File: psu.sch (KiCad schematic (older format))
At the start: 64 parts, among them J1 Screw_Terminal_01x02, J2 Barrel_Jack, J3 Binding posts, SW1 SW_SP4T, SW2 SW_SP4T, SW3 Lever toggle, U1 LM4040DBZ-2.5, U2 LT3081, U3 LM393, U4 LM334M, U5 LM317L_TO92, U6 LM317L_TO92

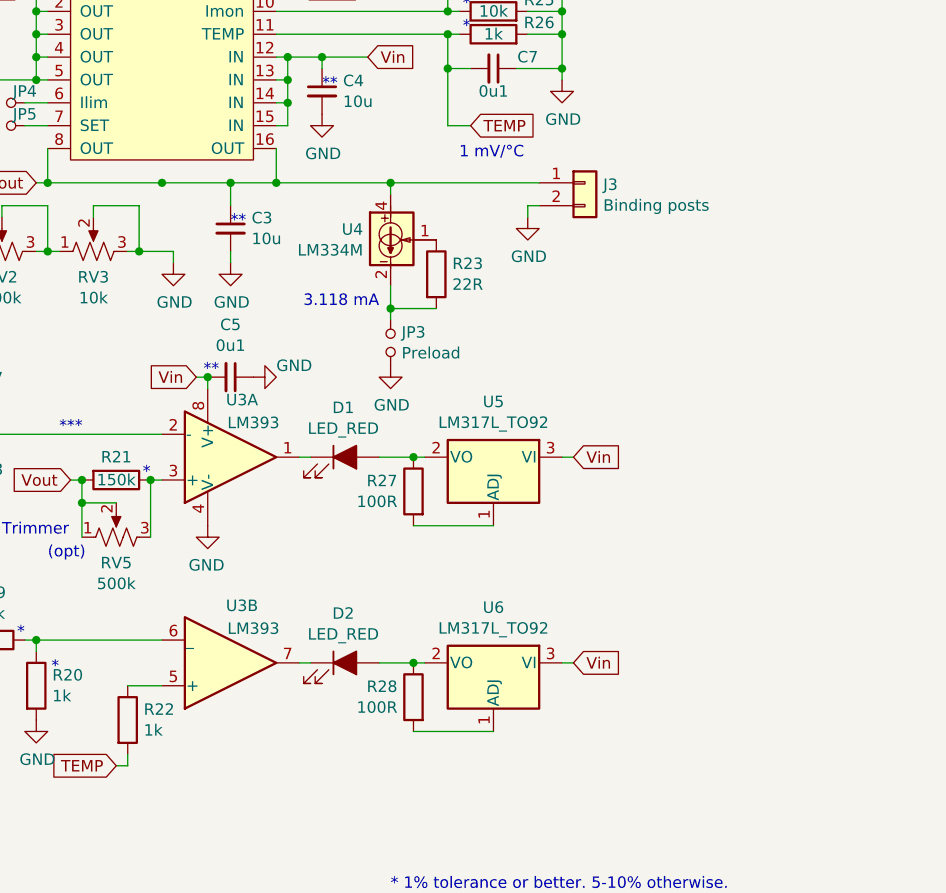
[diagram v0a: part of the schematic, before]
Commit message: More routing; some issues
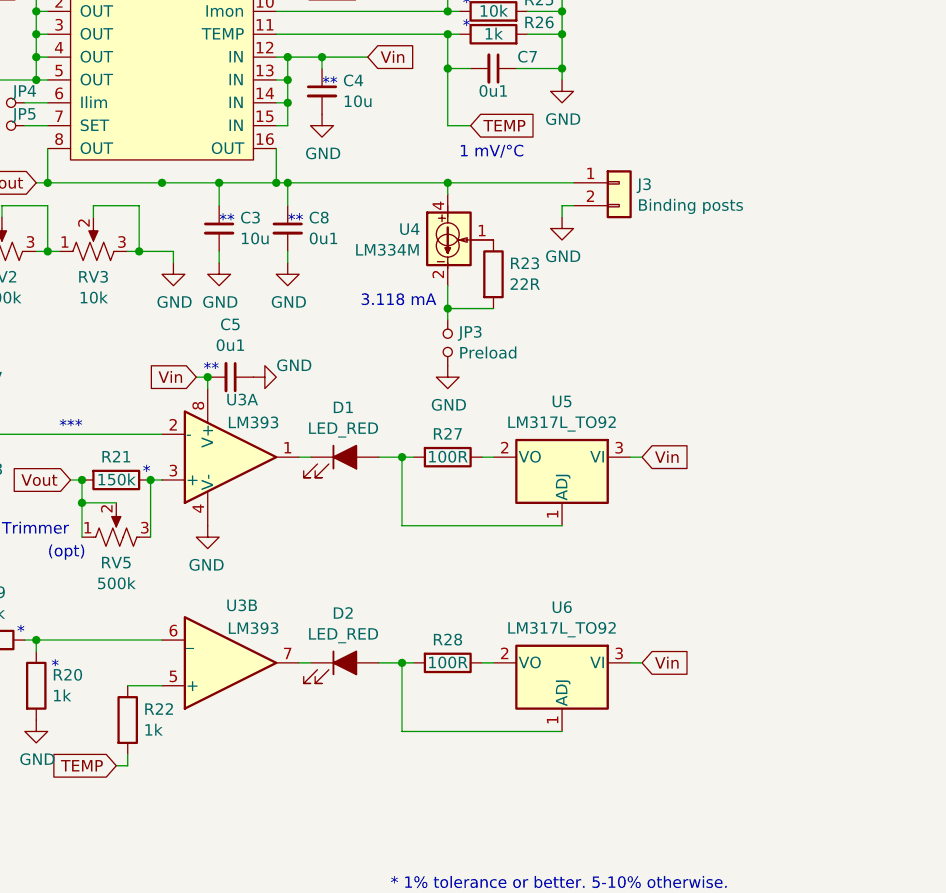
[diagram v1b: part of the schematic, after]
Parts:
- added C8: 0u1, Capacitor_THT:C_Disc_D5.0mm_W2.5mm_P2.50mm, symbol Device:C_Small
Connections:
- net GND: now also C8.2
- net Vout: now also C8.1
- net at R27.2, U5.1 (ADJ): now also D1.2 (A)
- net at R27.1, U5.2 (VO): no longer D1.2 (A)
- net at R28.2, U6.1 (ADJ): now also D2.2 (A)
- net at R28.1, U6.2 (VO): no longer D2.2 (A)
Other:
- moved on the sheet: C3, J3, JP3, R23, U4, U5

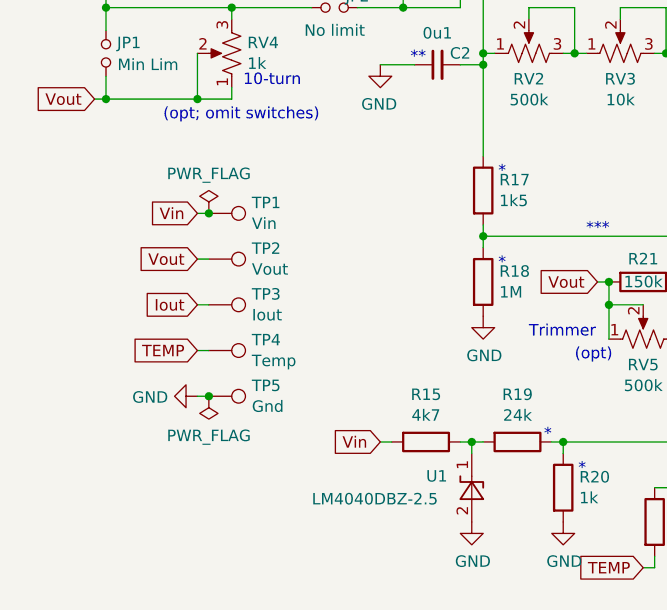
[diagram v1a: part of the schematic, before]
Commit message: It's all connected man
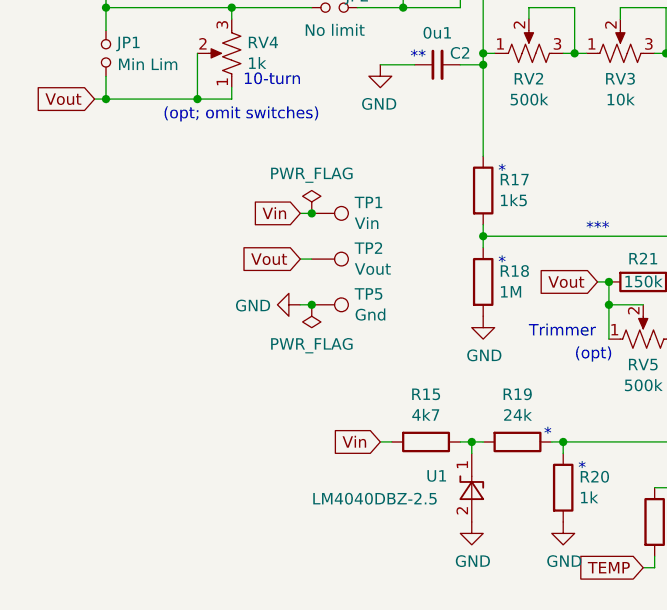
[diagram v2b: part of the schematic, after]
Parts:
- removed TP3: Iout, TestPoint:TestPoint_Bridge_Pitch2.54mm_Drill1.3mm, symbol Connector:TestPoint
- removed TP4: Temp, TestPoint:TestPoint_Bridge_Pitch2.54mm_Drill1.3mm, symbol Connector:TestPoint
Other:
- moved on the sheet: TP1, TP2, TP5
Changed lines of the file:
@@
 Wire Wire Line
 	7750 3650 7800 3650
-Text GLabel 3850 4550 0    50   Input ~ 0
+Text GLabel 4300 4550 0    50   Input ~ 0
 Vin
 Wire Wire Line
-	3850 4550 3900 4550
-Text GLabel 3850 5150 0    50   Input ~ 0
-TEMP
-Text GLabel 3850 4950 0    50   Input ~ 0
-Iout
-Text GLabel 3850 4750 0    50   Input ~ 0
+	4300 4550 4350 4550
+Text GLabel 4300 4750 0    50   Input ~ 0
 Vout
 Wire Wire Line
-	3850 4750 3900 4750
-Wire Wire Line
-	3900 4950 3850 4950
-Wire Wire Line
-	3850 5150 3900 5150
+	4300 4750 4350 4750
 Connection ~ 5100 3850
 $Comp
@@
 L Connector:TestPoint TP2
 U 1 1 5D1B06FD
-P 3900 4750
-F 0 "TP2" V 3854 4938 50  0000 L CNN
-F 1 "Vout" V 3945 4938 50  0000 L CNN
-F 2 "TestPoint:TestPoint_Bridge_Pitch2.54mm_Drill1.3mm" H 4100 4750 50  0001 C CNN
-F 3 "~" H 4100 4750 50  0001 C CNN
-	1    3900 4750
-	0    1    1    0
-$EndComp
-$Comp
-L Connector:TestPoint TP3
-U 1 1 5D1BB2CF
-P 3900 4950
-F 0 "TP3" V 3854 5138 50  0000 L CNN
-F 1 "Iout" V 3945 5138 50  0000 L CNN
-F 2 "TestPoint:TestPoint_Bridge_Pitch2.54mm_Drill1.3mm" H 4100 4950 50  0001 C CNN
-F 3 "~" H 4100 4950 50  0001 C CNN
-	1    3900 4950
-	0    1    1    0
-$EndComp
-$Comp
-L Connector:TestPoint TP4
-U 1 1 5D1BFE83
-P 3900 5150
-F 0 "TP4" V 3854 5338 50  0000 L CNN
-F 1 "Temp" V 3945 5338 50  0000 L CNN
-F 2 "TestPoint:TestPoint_Bridge_Pitch2.54mm_Drill1.3mm" H 4100 5150 50  0001 C CNN
-F 3 "~" H 4100 5150 50  0001 C CNN
-	1    3900 5150
+P 4350 4750
+F 0 "TP2" V 4304 4938 50  0000 L CNN
+F 1 "Vout" V 4395 4938 50  0000 L CNN
+F 2 "TestPoint:TestPoint_Bridge_Pitch2.54mm_Drill1.3mm" H 4550 4750 50  0001 C CNN
+F 3 "~" H 4550 4750 50  0001 C CNN
+	1    4350 4750
 	0    1    1    0
 $EndComp
@@
 L Connector:TestPoint TP1
 U 1 1 5D1C006B
-P 3900 4550
-F 0 "TP1" V 3854 4738 50  0000 L CNN
-F 1 "Vin" V 3945 4738 50  0000 L CNN
-F 2 "TestPoint:TestPoint_Bridge_Pitch2.54mm_Drill1.3mm" H 4100 4550 50  0001 C CNN
-F 3 "~" H 4100 4550 50  0001 C CNN
-	1    3900 4550
-	0    1    1    0
-$EndComp
-$Comp
-L power:GND #PWR01
-U 1 1 5D1D360C
-P 3850 5350
-F 0 "#PWR01" H 3850 5100 50  0001 C CNN
-F 1 "GND" V 3855 5222 50  0000 R CNN
-F 2 "" H 3850 5350 50  0001 C CNN
-F 3 "" H 3850 5350 50  0001 C CNN
-	1    3850 5350
-	0    1    1    0
-$EndComp
-Wire Wire Line
-	3850 5350 3900 5350
+P 4350 4550
+F 0 "TP1" V 4304 4738 50  0000 L CNN
+F 1 "Vin" V 4395 4738 50  0000 L CNN
+F 2 "TestPoint:TestPoint_Bridge_Pitch2.54mm_Drill1.3mm" H 4550 4550 50  0001 C CNN
+F 3 "~" H 4550 4550 50  0001 C CNN
+	1    4350 4550
+	0    1    1    0
+$EndComp
+Wire Wire Line
+	4300 4950 4350 4950
 $Comp
 L Connector:TestPoint TP5
 U 1 1 5D1D96AA
-P 3900 5350
-F 0 "TP5" V 3854 5538 50  0000 L CNN
-F 1 "Gnd" V 3945 5538 50  0000 L CNN
-F 2 "TestPoint:TestPoint_Bridge_Pitch2.54mm_Drill1.3mm" H 4100 5350 50  0001 C CNN
-F 3 "~" H 4100 5350 50  0001 C CNN
-	1    3900 5350
+P 4350 4950
+F 0 "TP5" V 4304 5138 50  0000 L CNN
+F 1 "Gnd" V 4395 5138 50  0000 L CNN
+F 2 "TestPoint:TestPoint_Bridge_Pitch2.54mm_Drill1.3mm" H 4550 4950 50  0001 C CNN
+F 3 "~" H 4550 4950 50  0001 C CNN
+	1    4350 4950
 	0    1    1    0
 $EndComp
@@
 L power:PWR_FLAG #FLG01
 U 1 1 5D1E24E0
-P 3900 4550
-F 0 "#FLG01" H 3900 4625 50  0001 C CNN
-F 1 "PWR_FLAG" H 3900 4723 50  0000 C CNN
-F 2 "" H 3900 4550 50  0001 C CNN
-F 3 "~" H 3900 4550 50  0001 C CNN
-	1    3900 4550
-	1    0    0    -1
-$EndComp
-Connection ~ 3900 4550
+P 4350 4550
+F 0 "#FLG01" H 4350 4625 50  0001 C CNN
+F 1 "PWR_FLAG" H 4350 4723 50  0000 C CNN
+F 2 "" H 4350 4550 50  0001 C CNN
+F 3 "~" H 4350 4550 50  0001 C CNN
+	1    4350 4550
+	1    0    0    -1
+$EndComp
+Connection ~ 4350 4550
 $Comp
 L power:PWR_FLAG #FLG02
 U 1 1 5D1E310A
-P 3900 5350
-F 0 "#FLG02" H 3900 5425 50  0001 C CNN
-F 1 "PWR_FLAG" H 3900 5523 50  0000 C CNN
-F 2 "" H 3900 5350 50  0001 C CNN
-F 3 "~" H 3900 5350 50  0001 C CNN
-	1    3900 5350
+P 4350 4950
+F 0 "#FLG02" H 4350 5025 50  0001 C CNN
+F 1 "PWR_FLAG" H 4350 5123 50  0000 C CNN
+F 2 "" H 4350 4950 50  0001 C CNN
+F 3 "~" H 4350 4950 50  0001 C CNN
+	1    4350 4950
 	-1   0    0    1
 $EndComp
-Connection ~ 3900 5350
+Connection ~ 4350 4950
 Wire Wire Line
 	5050 5550 5100 5550
@@
 Wire Wire Line
 	7050 5650 7100 5650
+$Comp
+L power:GND #PWR01
+U 1 1 5D1D360C
+P 4300 4950
+F 0 "#PWR01" H 4300 4700 50  0001 C CNN
+F 1 "GND" V 4305 4822 50  0000 R CNN
+F 2 "" H 4300 4950 50  0001 C CNN
+F 3 "" H 4300 4950 50  0001 C CNN
+	1    4300 4950
+	0    1    1    0
+$EndComp
 $EndSCHEMATC
